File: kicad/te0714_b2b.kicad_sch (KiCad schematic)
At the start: 3 parts

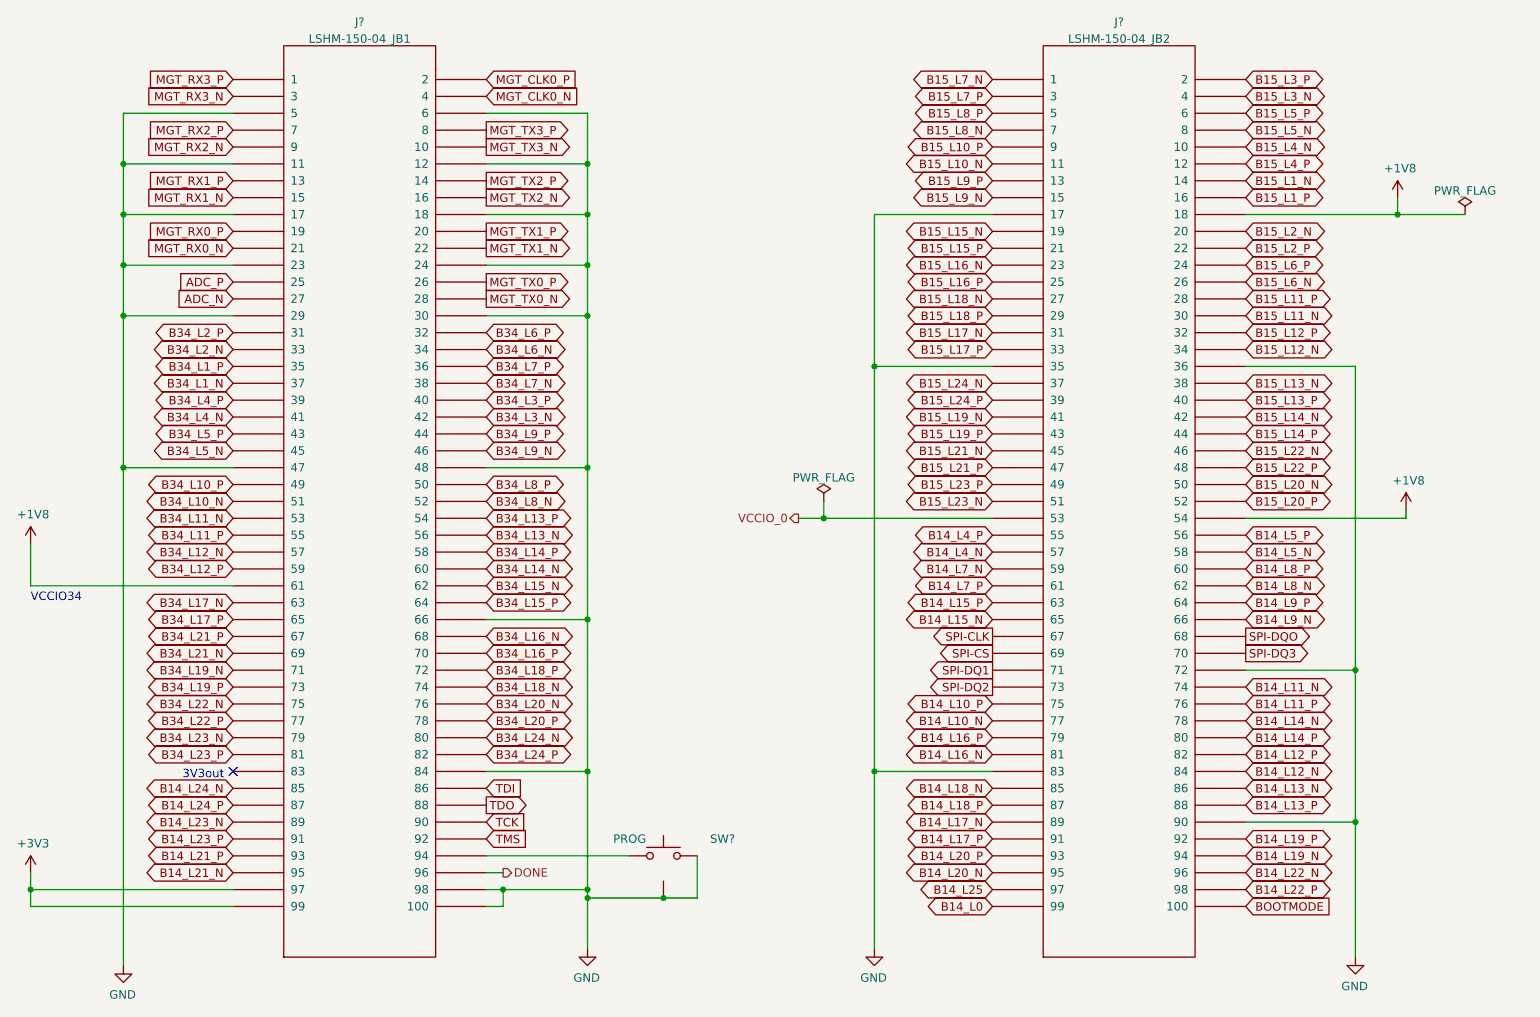
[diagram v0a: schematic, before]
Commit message: WIP
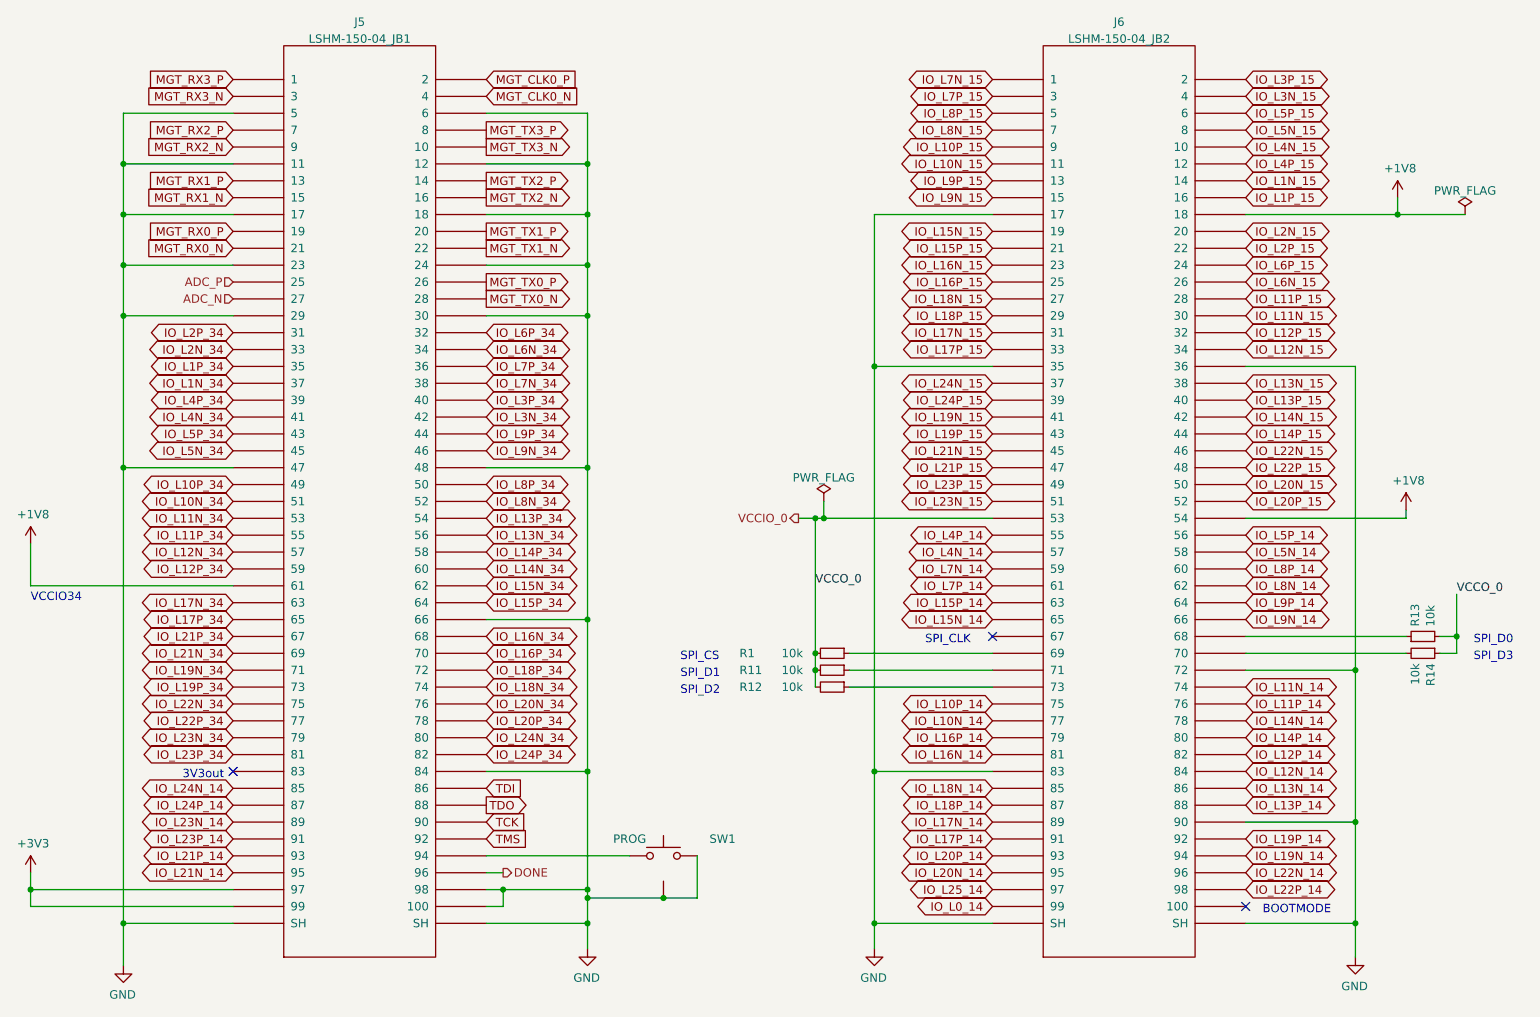
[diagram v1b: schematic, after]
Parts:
- added R1, R11, R12, R13, R14: 10k, Resistor_SMD:R_0603_1608Metric, symbol Device:R_Small
- J5, J6: renamed from J?; footprint MODULE -> Connector_Samtec:Samtec_LSHM-150-xx.x-x-DV-S_2x50-1SH_P0.50mm_Vertical
- gave numbers to parts that had none: 1
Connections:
- net GND: now also J5.SH, J6.SH
- net VCCIO_0: now also R1.2, R11.2, R12.2, R13.2, R14.1
- net B14_L0 renamed IO_L0_14
- net B14_L10_N renamed IO_L10N_14
- net B14_L10_P renamed IO_L10P_14
- net B14_L11_N renamed IO_L11N_14
- net B14_L11_P renamed IO_L11P_14
- net B14_L12_N renamed IO_L12N_14
- net B14_L12_P renamed IO_L12P_14
- net B14_L13_N renamed IO_L13N_14
- net B14_L13_P renamed IO_L13P_14
- net B14_L14_N renamed IO_L14N_14
- net B14_L14_P renamed IO_L14P_14
- net B14_L15_N renamed IO_L15N_14
- net B14_L15_P renamed IO_L15P_14
- net B14_L16_N renamed IO_L16N_14
- net B14_L16_P renamed IO_L16P_14
- net B14_L17_N renamed IO_L17N_14
- net B14_L17_P renamed IO_L17P_14
- net B14_L18_N renamed IO_L18N_14
- net B14_L18_P renamed IO_L18P_14
- net B14_L19_N renamed IO_L19N_14
- net B14_L19_P renamed IO_L19P_14
- net B14_L20_N renamed IO_L20N_14
- net B14_L20_P renamed IO_L20P_14
- net B14_L21_N renamed IO_L21N_14
- net B14_L21_P renamed IO_L21P_14
- net B14_L22_N renamed IO_L22N_14
- net B14_L22_P renamed IO_L22P_14
- net B14_L23_N renamed IO_L23N_14
- net B14_L23_P renamed IO_L23P_14
- net B14_L24_N renamed IO_L24N_14
- net B14_L24_P renamed IO_L24P_14
- net B14_L25 renamed IO_L25_14
- net B14_L4_N renamed IO_L4N_14
- net B14_L4_P renamed IO_L4P_14
- net B14_L5_N renamed IO_L5N_14
- net B14_L5_P renamed IO_L5P_14
- net B14_L7_N renamed IO_L7N_14
- net B14_L7_P renamed IO_L7P_14
- net B14_L8_N renamed IO_L8N_14
- net B14_L8_P renamed IO_L8P_14
- net B14_L9_N renamed IO_L9N_14
- net B14_L9_P renamed IO_L9P_14
- net B15_L10_N renamed IO_L10N_15
- net B15_L10_P renamed IO_L10P_15
- net B15_L11_N renamed IO_L11N_15
- net B15_L11_P renamed IO_L11P_15
- net B15_L12_N renamed IO_L12N_15
- net B15_L12_P renamed IO_L12P_15
- net B15_L13_N renamed IO_L13N_15
- net B15_L13_P renamed IO_L13P_15
- net B15_L14_N renamed IO_L14N_15
- net B15_L14_P renamed IO_L14P_15
- net B15_L15_N renamed IO_L15N_15
- net B15_L15_P renamed IO_L15P_15
- net B15_L16_N renamed IO_L16N_15
- net B15_L16_P renamed IO_L16P_15
- net B15_L17_N renamed IO_L17N_15
- net B15_L17_P renamed IO_L17P_15
- net B15_L18_N renamed IO_L18N_15
- net B15_L18_P renamed IO_L18P_15
- net B15_L19_N renamed IO_L19N_15
- net B15_L19_P renamed IO_L19P_15
- net B15_L1_N renamed IO_L1N_15
- net B15_L1_P renamed IO_L1P_15
- net B15_L20_N renamed IO_L20N_15
- net B15_L20_P renamed IO_L20P_15
- net B15_L21_N renamed IO_L21N_15
- net B15_L21_P renamed IO_L21P_15
- net B15_L22_N renamed IO_L22N_15
- net B15_L22_P renamed IO_L22P_15
- net B15_L23_N renamed IO_L23N_15
- net B15_L23_P renamed IO_L23P_15
- net B15_L24_N renamed IO_L24N_15
- net B15_L24_P renamed IO_L24P_15
- net B15_L2_N renamed IO_L2N_15
- net B15_L2_P renamed IO_L2P_15
- net B15_L3_N renamed IO_L3N_15
- net B15_L3_P renamed IO_L3P_15
- net B15_L4_N renamed IO_L4N_15
- net B15_L4_P renamed IO_L4P_15
- net B15_L5_N renamed IO_L5N_15
- net B15_L5_P renamed IO_L5P_15
- net B15_L6_N renamed IO_L6N_15
- net B15_L6_P renamed IO_L6P_15
- net B15_L7_N renamed IO_L7N_15
- net B15_L7_P renamed IO_L7P_15
- net B15_L8_N renamed IO_L8N_15
- net B15_L8_P renamed IO_L8P_15
- net B15_L9_N renamed IO_L9N_15
- net B15_L9_P renamed IO_L9P_15
- net B34_L10_N renamed IO_L10N_34
- net B34_L10_P renamed IO_L10P_34
- net B34_L11_N renamed IO_L11N_34
- net B34_L11_P renamed IO_L11P_34
- net B34_L12_N renamed IO_L12N_34
- net B34_L12_P renamed IO_L12P_34
- net B34_L13_N renamed IO_L13N_34
- net B34_L13_P renamed IO_L13P_34
- net B34_L14_N renamed IO_L14N_34
- net B34_L14_P renamed IO_L14P_34
- net B34_L15_N renamed IO_L15N_34
- net B34_L15_P renamed IO_L15P_34
- net B34_L16_N renamed IO_L16N_34
- net B34_L16_P renamed IO_L16P_34
- net B34_L17_N renamed IO_L17N_34
- net B34_L17_P renamed IO_L17P_34
- net B34_L18_N renamed IO_L18N_34
- net B34_L18_P renamed IO_L18P_34
- net B34_L19_N renamed IO_L19N_34
- net B34_L19_P renamed IO_L19P_34
- net B34_L1_N renamed IO_L1N_34
- net B34_L1_P renamed IO_L1P_34
- net B34_L20_N renamed IO_L20N_34
- net B34_L20_P renamed IO_L20P_34
- net B34_L21_N renamed IO_L21N_34
- net B34_L21_P renamed IO_L21P_34
- net B34_L22_N renamed IO_L22N_34
- net B34_L22_P renamed IO_L22P_34
- net B34_L23_N renamed IO_L23N_34
- net B34_L23_P renamed IO_L23P_34
- net B34_L24_N renamed IO_L24N_34
- net B34_L24_P renamed IO_L24P_34
- net B34_L2_N renamed IO_L2N_34
- net B34_L2_P renamed IO_L2P_34
- net B34_L3_N renamed IO_L3N_34
- net B34_L3_P renamed IO_L3P_34
- net B34_L4_N renamed IO_L4N_34
- net B34_L4_P renamed IO_L4P_34
- net B34_L5_N renamed IO_L5N_34
- net B34_L5_P renamed IO_L5P_34
- net B34_L6_N renamed IO_L6N_34
- net B34_L6_P renamed IO_L6P_34
- net B34_L7_N renamed IO_L7N_34
- net B34_L7_P renamed IO_L7P_34
- net B34_L8_N renamed IO_L8N_34
- net B34_L8_P renamed IO_L8P_34
- net B34_L9_N renamed IO_L9N_34
- net B34_L9_P renamed IO_L9P_34
- net BOOTMODE: no longer names the net of J6.100
- net SPI-CLK: no longer names the net of J6.67
- net SPI-CS: no longer names the net of J6.69
- net SPI-CS: now also R1.1
- net SPI-DQ1: no longer names the net of J6.71
- net SPI-DQ1: now also R11.1
- net SPI-DQ2: no longer names the net of J6.73
- net SPI-DQ2: now also R12.1
- net SPI-DQ3: no longer names the net of J6.70
- net SPI-DQ3: now also R14.2
- net SPI-DQO: no longer names the net of J6.68
- net SPI-DQO: now also R13.1
- no-connect marks 1 -> 3
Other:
- note added: "BOOTMODE"
- note added: "SPI_CLK"
- note added: "SPI_CS"
- note added: "SPI_D0"
- note added: "SPI_D1"
- note added: "SPI_D2"
- note added: "SPI_D3"
